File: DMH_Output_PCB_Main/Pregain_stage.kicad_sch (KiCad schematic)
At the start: 9 parts, among them U7 TL072

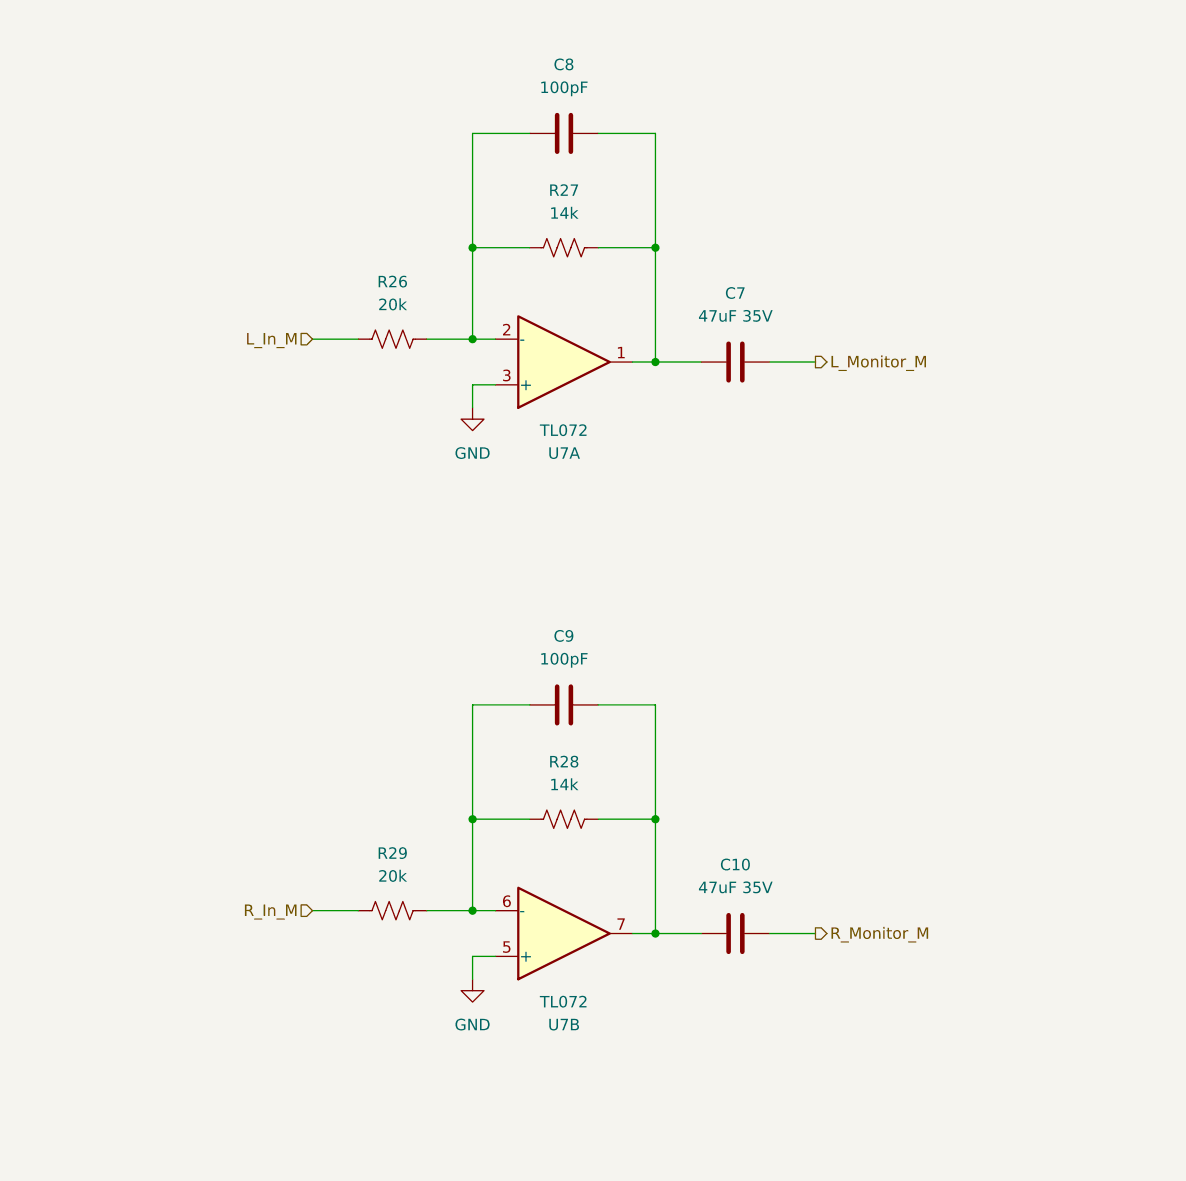
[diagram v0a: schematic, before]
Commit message: Prepped for Main PCB design
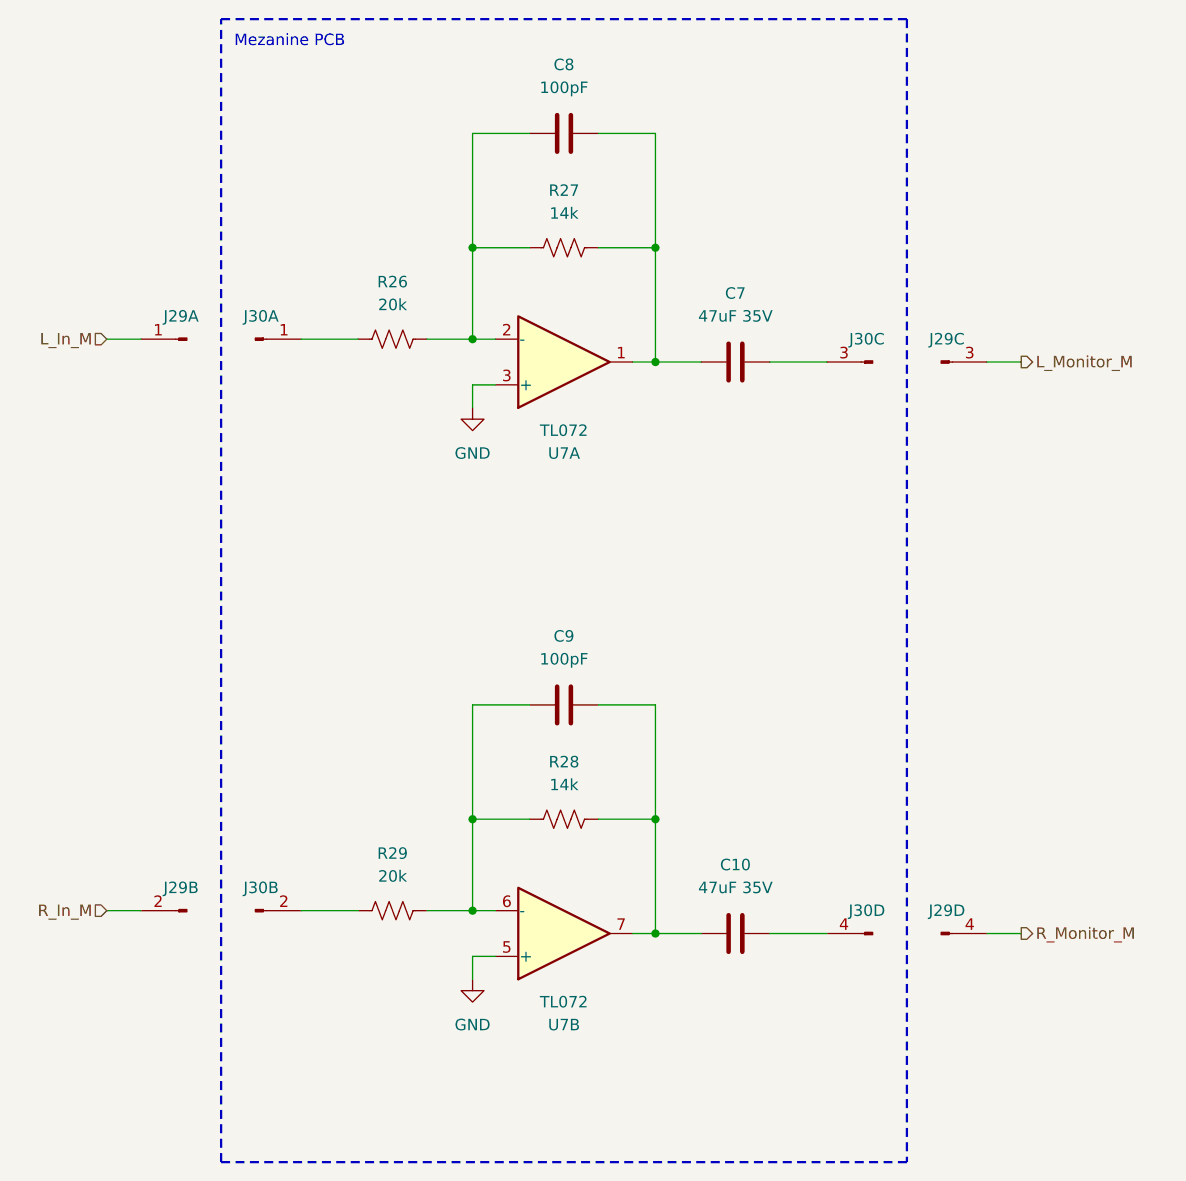
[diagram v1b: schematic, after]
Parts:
- added J29: Conn_01x04_PinHeader, Connector_PinSocket_2.54mm:PinSocket_1x04_P2.54mm_Vertical, symbol SynthStuff:Conn_01x04_PinHeader
- added J30: Conn_01x04_PinHeader, Connector_PinHeader_2.54mm:PinHeader_1x04_P2.54mm_Vertical, symbol SynthStuff:Conn_01x04_PinHeader
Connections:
- net L_In_M: now also J29.1 (Pin_1); no longer R26.1
- net L_Monitor_M: now also J29.3 (Pin_3); no longer C7.2
- net R_In_M: now also J29.2 (Pin_2); no longer R29.1
- net R_Monitor_M: now also J29.4 (Pin_4); no longer C10.2
- new net: C7.2, J30.3 (Pin_3)
- new net: J30.2 (Pin_2), R29.1
- new net: C10.2, J30.4 (Pin_4)
- new net: J30.1 (Pin_1), R26.1
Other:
- note added: "Mezanine PCB"
